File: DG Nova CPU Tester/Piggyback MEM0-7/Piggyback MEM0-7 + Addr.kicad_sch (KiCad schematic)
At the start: 24 parts, among them J1 Conn_02x18_Odd_Even, J22 Arduino Digital Pins, J23 Arduino Digital Pins, J3 Conn_01x17, SW1 Arduino Mega Reset, SW4 SW_DIP_x04, U1 74LS03, U2 74LS03, U3 74LS04, U4 74HC595, U5 74LS03, U6 74LS03, U7 74LS03, U8 74LS03, U9 74HC595

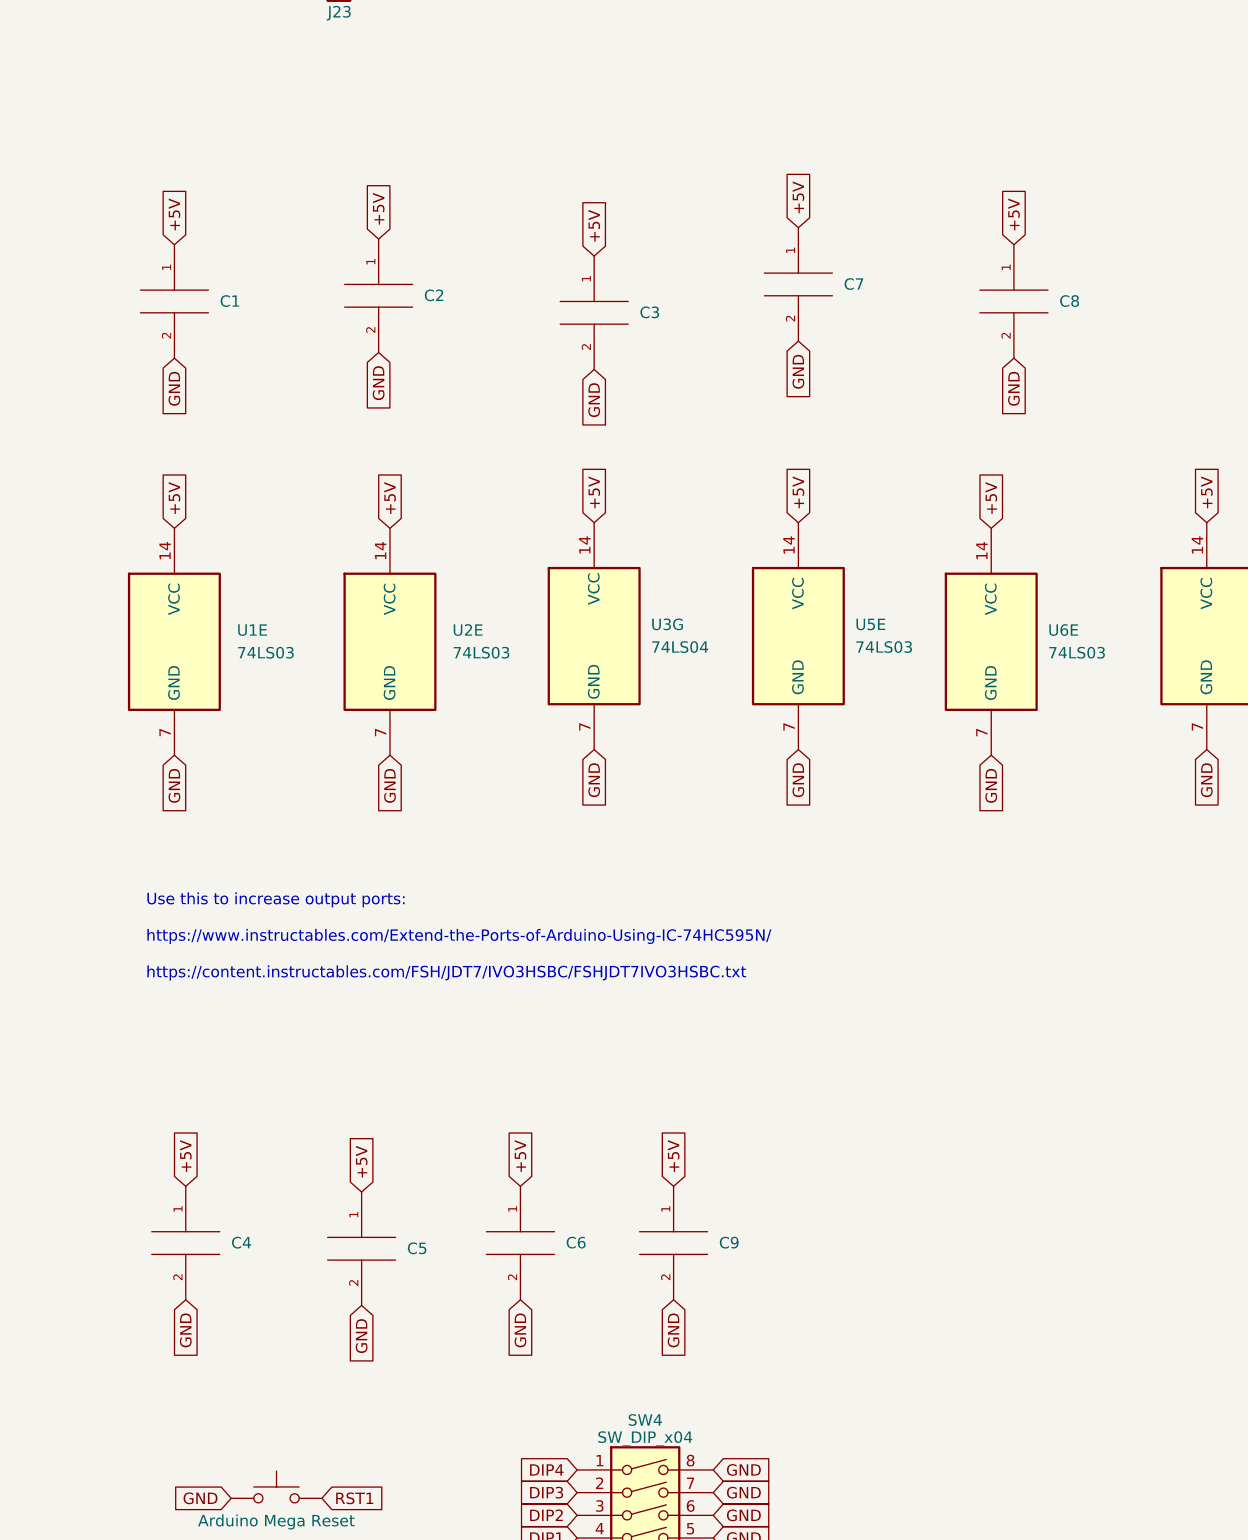
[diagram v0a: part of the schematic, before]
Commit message: more
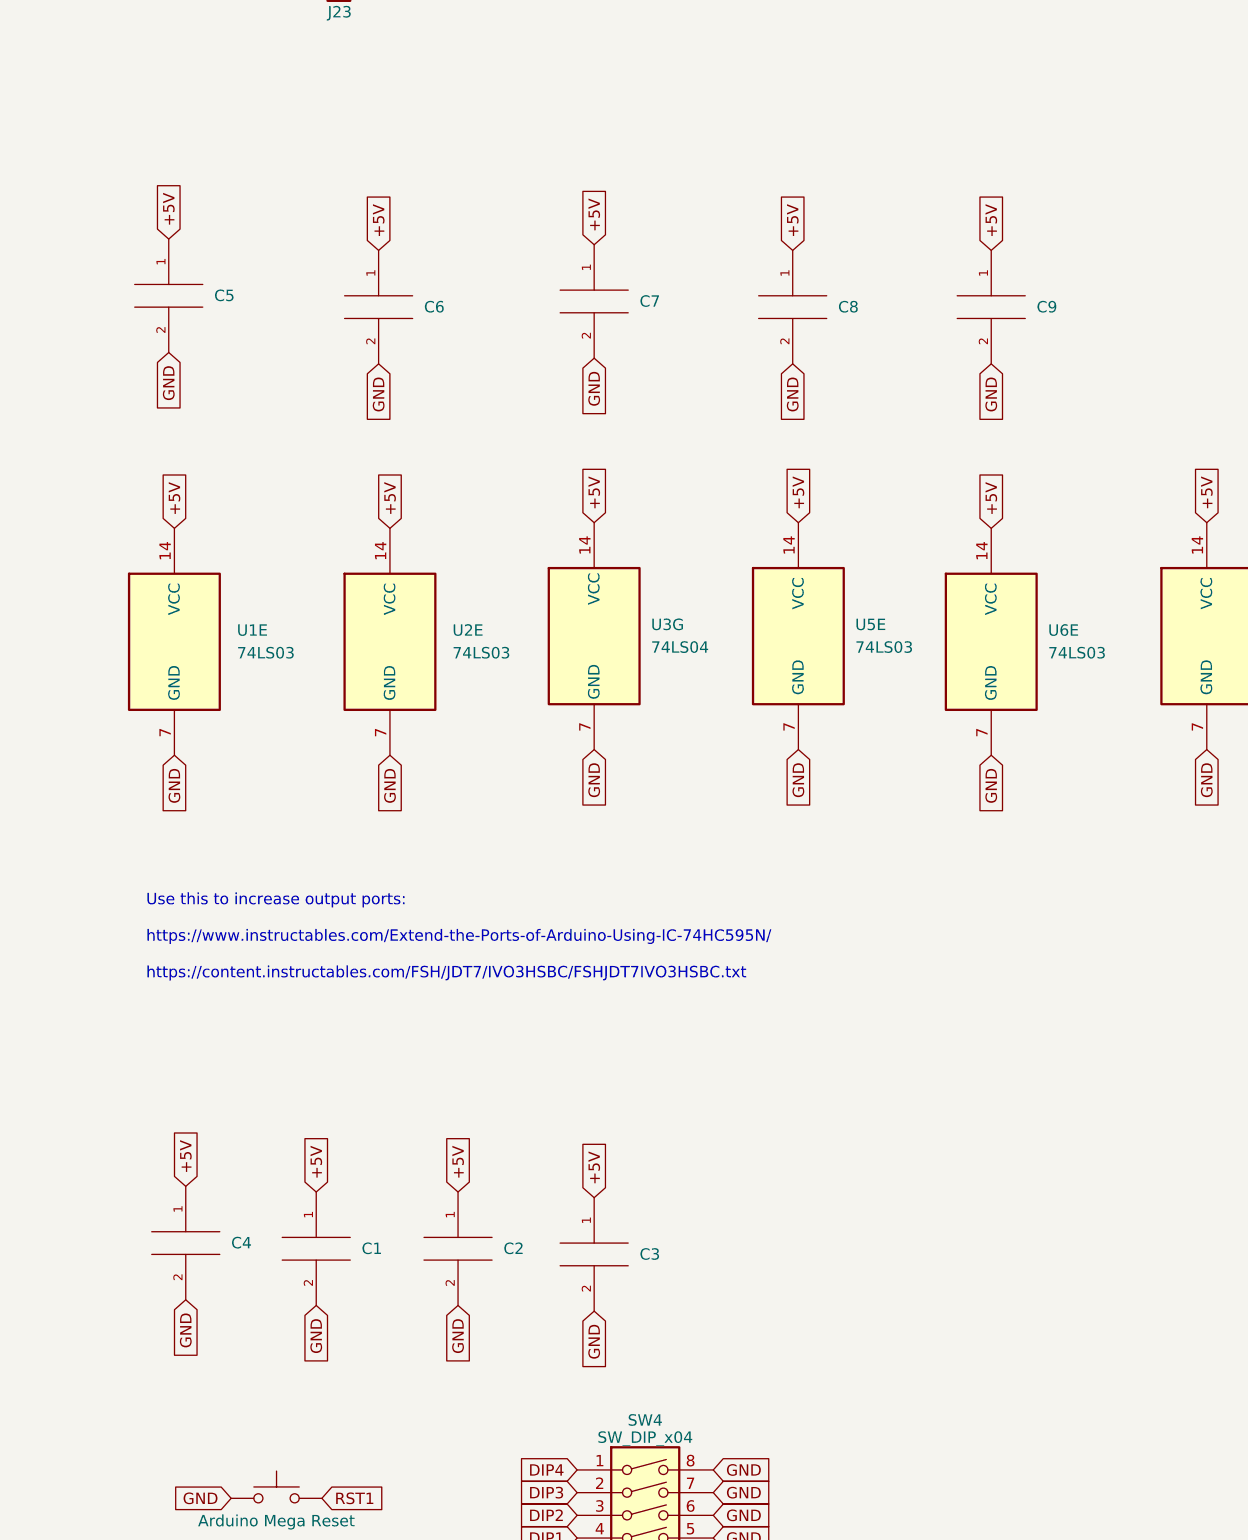
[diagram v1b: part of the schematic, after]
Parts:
- C1, C2, C3, C4, C5, C6, C7, C8, C9: footprint Forgotten Machines:Disc Capacitor Common Entrex Trapezoid -> Forgotten Machines:Disc Capacitor Entrex Trapezoid .10
